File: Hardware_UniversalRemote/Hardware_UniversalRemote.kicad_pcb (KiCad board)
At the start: 2 copper layers, 140 x 140 mm, 58 parts, among them J1 USB_B_Micro, Q1 S8050, Q2 BSS138, Q3 S8050, Q4 S8050, Q5 S8050, Q6 S8050, Q7 S8050, SW1 SW_Push, SW2 SW_Push, SW3 SW_Push, U1 ESP32-WROOM-32U, U2 LM1117T-3.3, U3 HS0038B, U4 CH340C

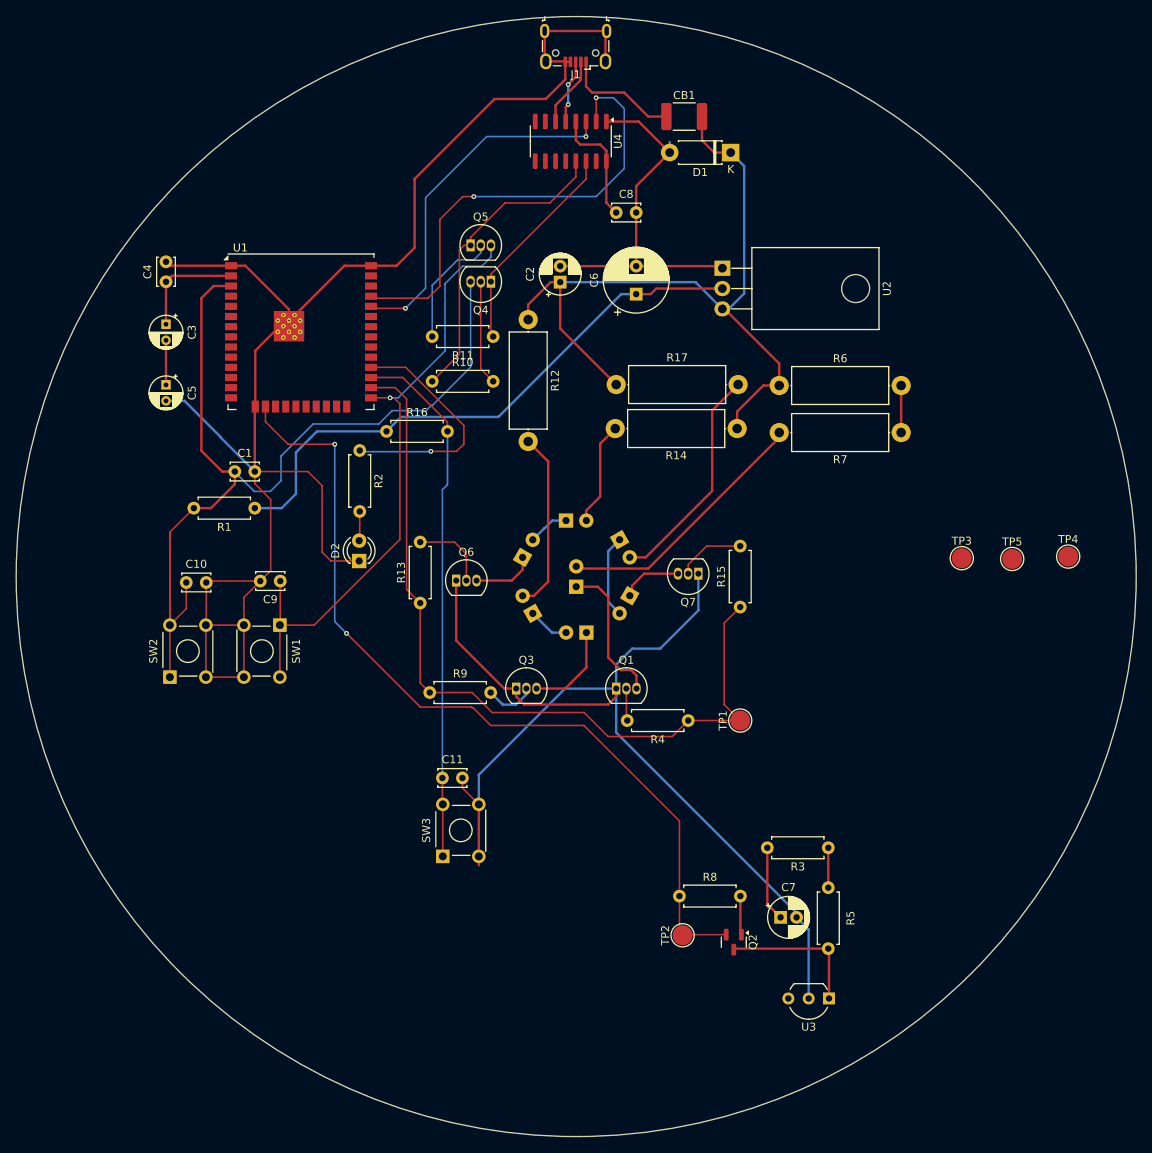
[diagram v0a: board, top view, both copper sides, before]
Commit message: add trace
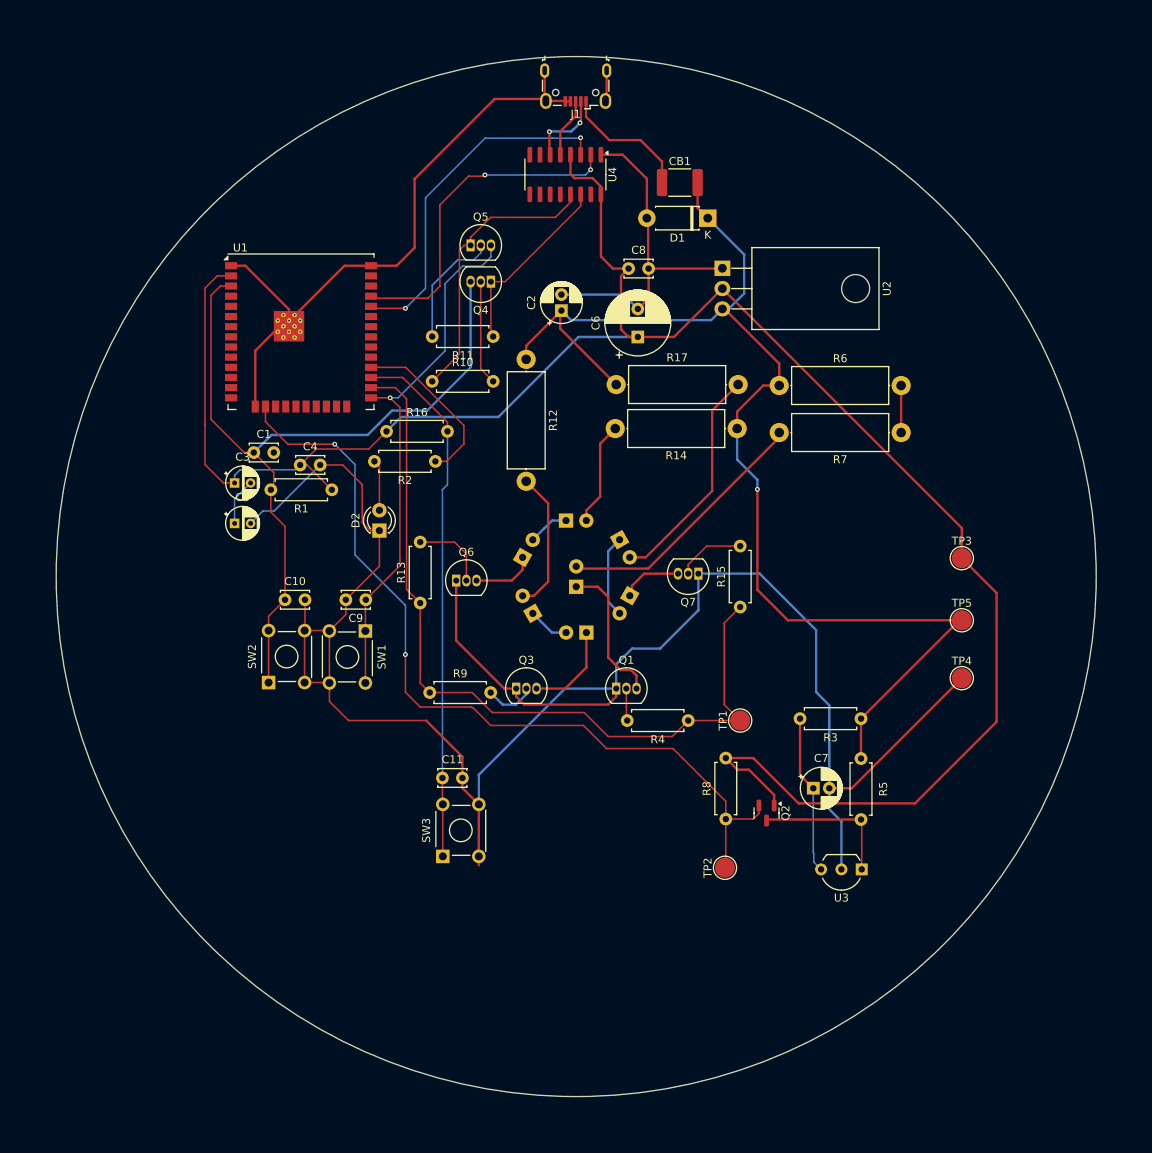
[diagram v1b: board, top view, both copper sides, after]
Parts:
- moved C4 28.4 mm to (76.5, 105.0), turned to 0 degrees
- moved C3 21.6 mm to (68.3, 107.3), turned to 0 degrees
- moved TP4 20.2 mm to (159.2, 131.7)
- moved C5 19.3 mm to (68.3, 112.3), turned to 0 degrees
- moved R3 16.7 mm to (146.6, 136.8)
- moved U3 16.7 mm to (146.7, 155.6)
- moved C7 16.7 mm to (140.6, 145.5)
- moved Q2 16.7 mm to (134.8, 148.6)
- moved R5 16.7 mm to (146.6, 149.4)
- moved C10 12.5 mm to (74.6, 121.9)
- moved SW2 12.4 mm to (72.5, 132.2)
- moved R8 11.2 mm to (129.7, 149.3), turned to 90 degrees
- moved C9 10.9 mm to (84.7, 121.9)
- moved SW1 10.7 mm to (84.7, 125.8)
- moved TP2 9.97 mm to (129.6, 155.4)
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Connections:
- C3 pad 1: Net-(U1-VDD) -> +3.3V
- C4 pad 1: Net-(U1-VDD) -> +3.3V
- U1 pad 2: Net-(U1-VDD) -> +3.3V
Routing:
- net +3.3V: track 93.8 -> 256.3 mm
- net +5V: track 99.8 -> 153.6 mm, vias 0 -> 1
- net /EN: track 126.3 -> 99.4 mm
- net GND: track 395.1 -> 378.6 mm
- net /TXD0: track 57.9 -> 42.0 mm
- net Net-(U1-VDD): track 13.7 -> 0.00 mm
- net /IO0: track 78.6 -> 66.6 mm
- net Net-(U3-VCC): track 9.39 -> 19.9 mm
- net /IO17: track 30.4 -> 21.4 mm, vias 1 -> 0
- net Net-(D4-A): track 22.5 -> 17.6 mm
- net /RTS: track 27.9 -> 24.5 mm
- net /DTR: track 38.7 -> 35.7 mm
- net Net-(D2-A): track 3.68 -> 6.37 mm
- net Net-(J1-VBUS): track 14.7 -> 16.4 mm
- net /IO13: track 107.2 -> 105.8 mm
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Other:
- board size 140 x 140 mm -> 130 x 130 mm
